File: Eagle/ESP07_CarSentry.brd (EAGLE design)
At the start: 21.6 x 27.7 mm, 45 parts, among them Q1 PFET, Q2 NPN or N-FET, Q3 PFET, Q4 NPN

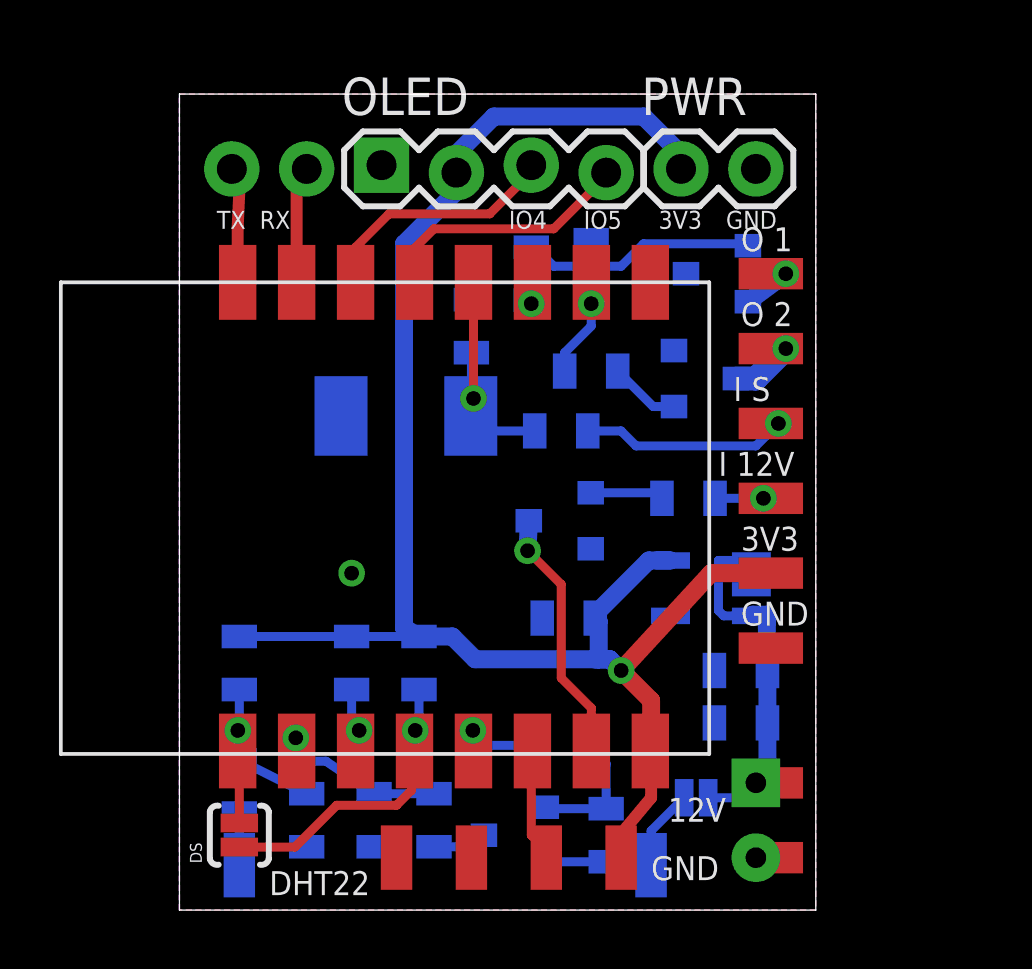
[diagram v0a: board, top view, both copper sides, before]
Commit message: rev 2 or something
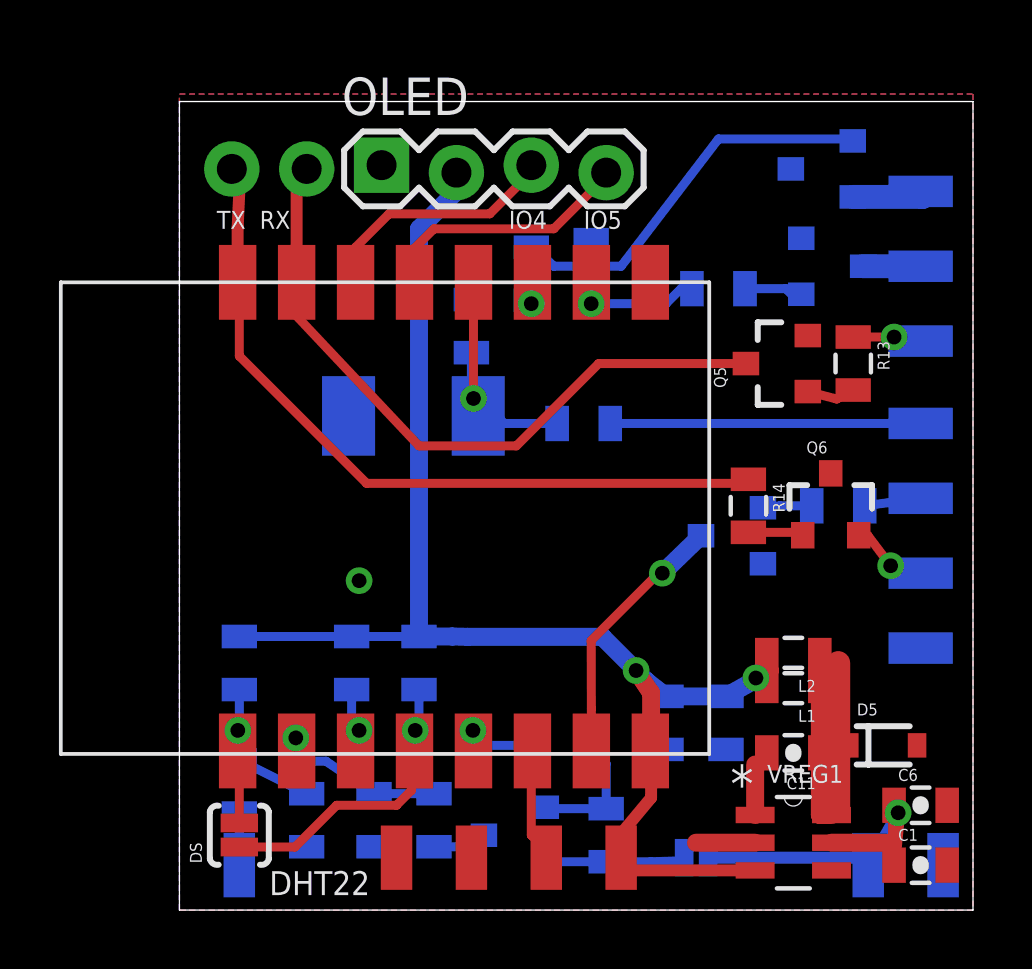
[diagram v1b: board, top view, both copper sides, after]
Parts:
- removed C2: (no value), SparkFun-Capacitors:CPOL-RADIAL-100UF-25V
- removed C3: 0.1uF, SparkFun-Capacitors:0805-CAP
- removed PWR: (no value), SparkFun-Connectors:1X02
- removed VREG: MCP1755T-330I/OT, Microchip_By_element14_Batch_1:SOT95P270X145-5N
- added C11, C6, C9: 0.1uF, SparkFun-Capacitors:0805-CAP
- added D5: BAT20J, SparkFun-DiscreteSemi:SOD-323
- added L1, L2: (no value), SparkFun-Passives:0805
- added Q5: NPN, SparkFun-DiscreteSemi:SOT23-3
- added Q6: PFET, SparkFun-DiscreteSemi:SOT23-3
- added R13: 4K7, SparkFun-Resistors:0805
- added R14: 1K, SparkFun-Resistors:0805
- added VREG1: LMR16006YQ3DDCRQ1, CuriousTech:SOT-23-6
- C1: value 0.1uF -> 2.2uF
- C4: value 1uF -> 10uF
- moved C1 14.6 mm to (25.1, 1.52), flipped to the top
- moved U$13 13.5 mm to (25.1, 11.4), turned to 0 degrees
- moved U$10 9.37 mm to (25.1, 19.3), flipped to the bottom
- moved Q4 5.86 mm to (18.8, 12.7)
- moved U$6 5.85 mm to (25.9, 1.52), flipped to the bottom, turned to 270 degrees
- moved U$3 5.80 mm to (25.1, 21.8), flipped to the bottom
- moved U$9 5.80 mm to (25.1, 24.4), flipped to the bottom
- moved Q2 5.76 mm to (22.1, 21.8)
- moved R9 5.14 mm to (18.3, 21.1)
- moved R12 5.09 mm to (22.4, 13.7)
- moved U$11 5.08 mm to (25.1, 8.89), flipped to the bottom
- moved U$14 5.08 mm to (25.1, 16.5), flipped to the bottom
- moved U$2 5.08 mm to (25.1, 14.0), flipped to the bottom
- moved Q3 5.03 mm to (21.8, 25.1)
- moved U$16 4.33 mm to (23.4, 1.52), flipped to the bottom, turned to 270 degrees
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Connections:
- removed net 12V: 12VA.2, C2.1, C3.1, C4.1, U$16.>NAME, VREG.1, VREG.3
- new net +12V: 12VA.2, C1.1, C6.1, U$16.>NAME, VREG1.5
- new net N$12: Q5.1, R13.2
- new net N$13: C11.1, D5.C, L1.1, L2.1, VREG1.6
- new net N$14: C11.2, VREG1.1
- new net N$15: R13.1, U$10.>NAME
- new net N$16: Q6.2, U$13.>NAME
- new net N$17: Q6.1, R14.2
- net 3V3: now also C4.1, C9.1, L1.2, L2.2, VREG1.3; no longer C1.1, PWR.1, U$10.>NAME, VREG.5
- net ADCHI: no longer U$13.>NAME
- net GND: now also C6.2, C9.2, D5.A, Q5.2, Q6.3, VREG1.2; no longer C2.2, C3.2, PWR.2, VREG.2
- net RXD: now also Q5.3
- net TXD: now also R14.1
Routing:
- net TXD: track 3.89 -> 25.5 mm
- net RXD: track 3.93 -> 23.4 mm
- net +12V: track 0.00 -> 15.9 mm, vias 0 -> 1
- net 12V: track 12.8 -> 0.00 mm
- net N$13: track 0.00 -> 12.2 mm
- net 3V3: track 60.1 -> 48.4 mm, vias 1 -> 2
- net N$2: track 7.96 -> 13.7 mm
- net N$5: track 7.25 -> 10.5 mm, vias 1 -> 0
- net N$16: track 0.00 -> 2.72 mm, vias 0 -> 1
- net N$15: track 0.00 -> 2.30 mm, vias 0 -> 1
- net N$14: track 0.00 -> 2.27 mm
- net GND: track 0.00 -> 2.01 mm
- net N$17: track 0.00 -> 1.89 mm
- net ADCHI: track 6.46 -> 4.76 mm
- net N$12: track 0.00 -> 1.65 mm
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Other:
- board size 21.6 x 27.7 mm -> 26.9 x 27.4 mm
- board text removed: "3V3"
